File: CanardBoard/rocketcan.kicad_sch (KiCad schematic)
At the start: 18 parts, among them J10 G125-MH104M4-04AD000P, U13 TCAN3413DDFR, U14 TPS2521

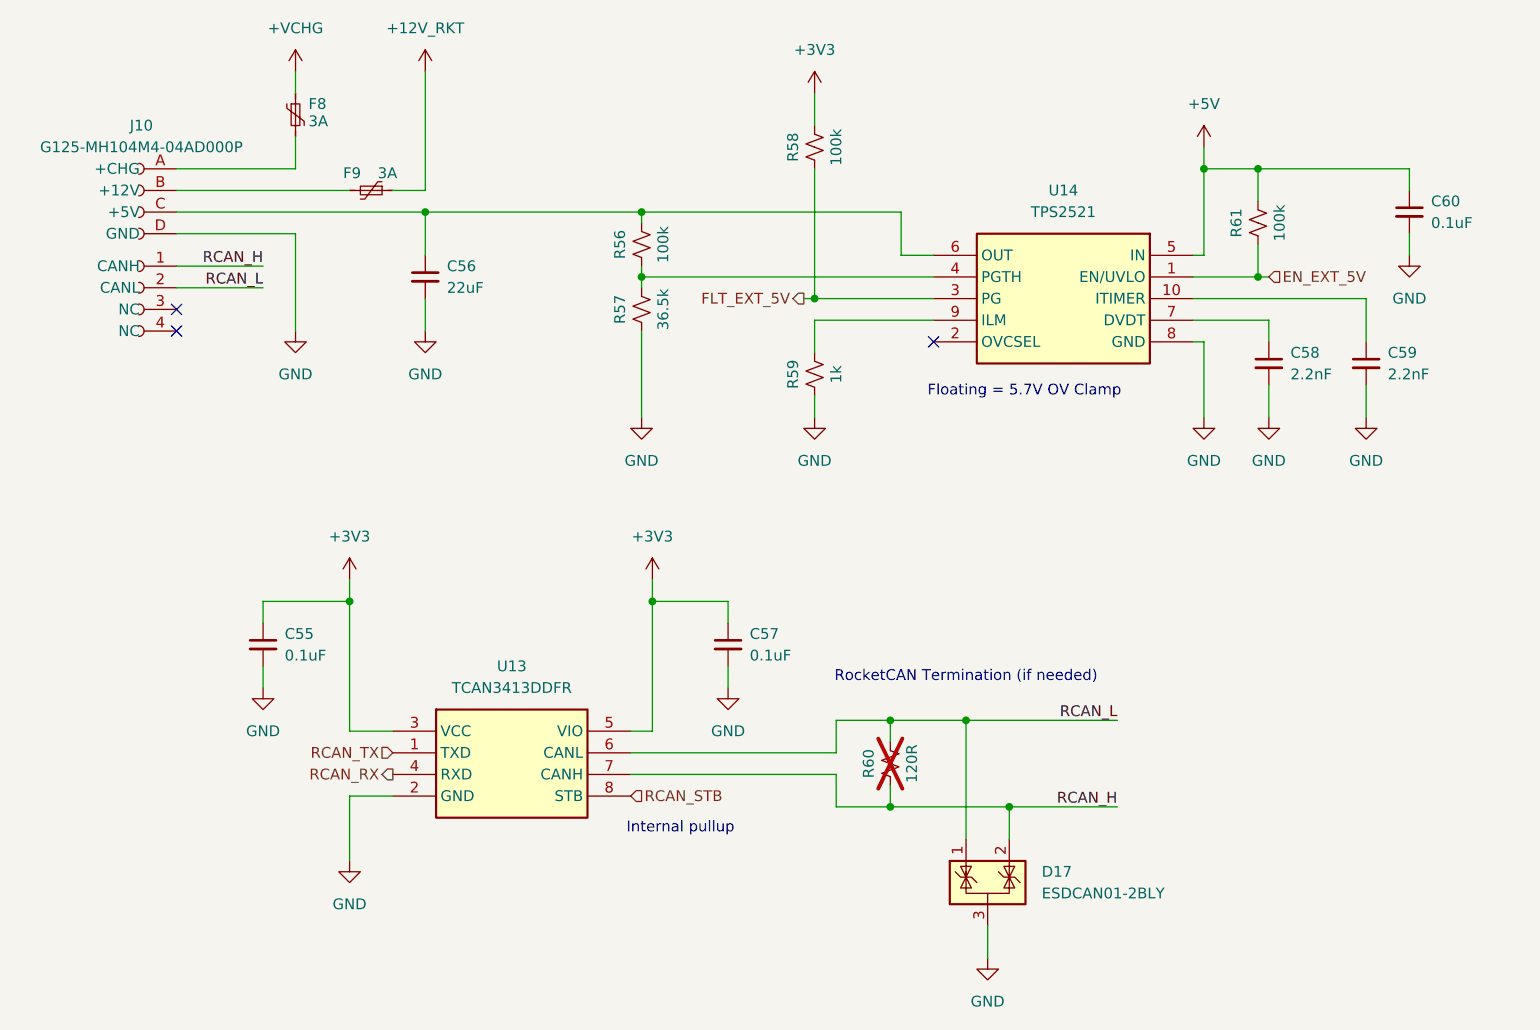
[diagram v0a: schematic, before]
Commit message: stuff
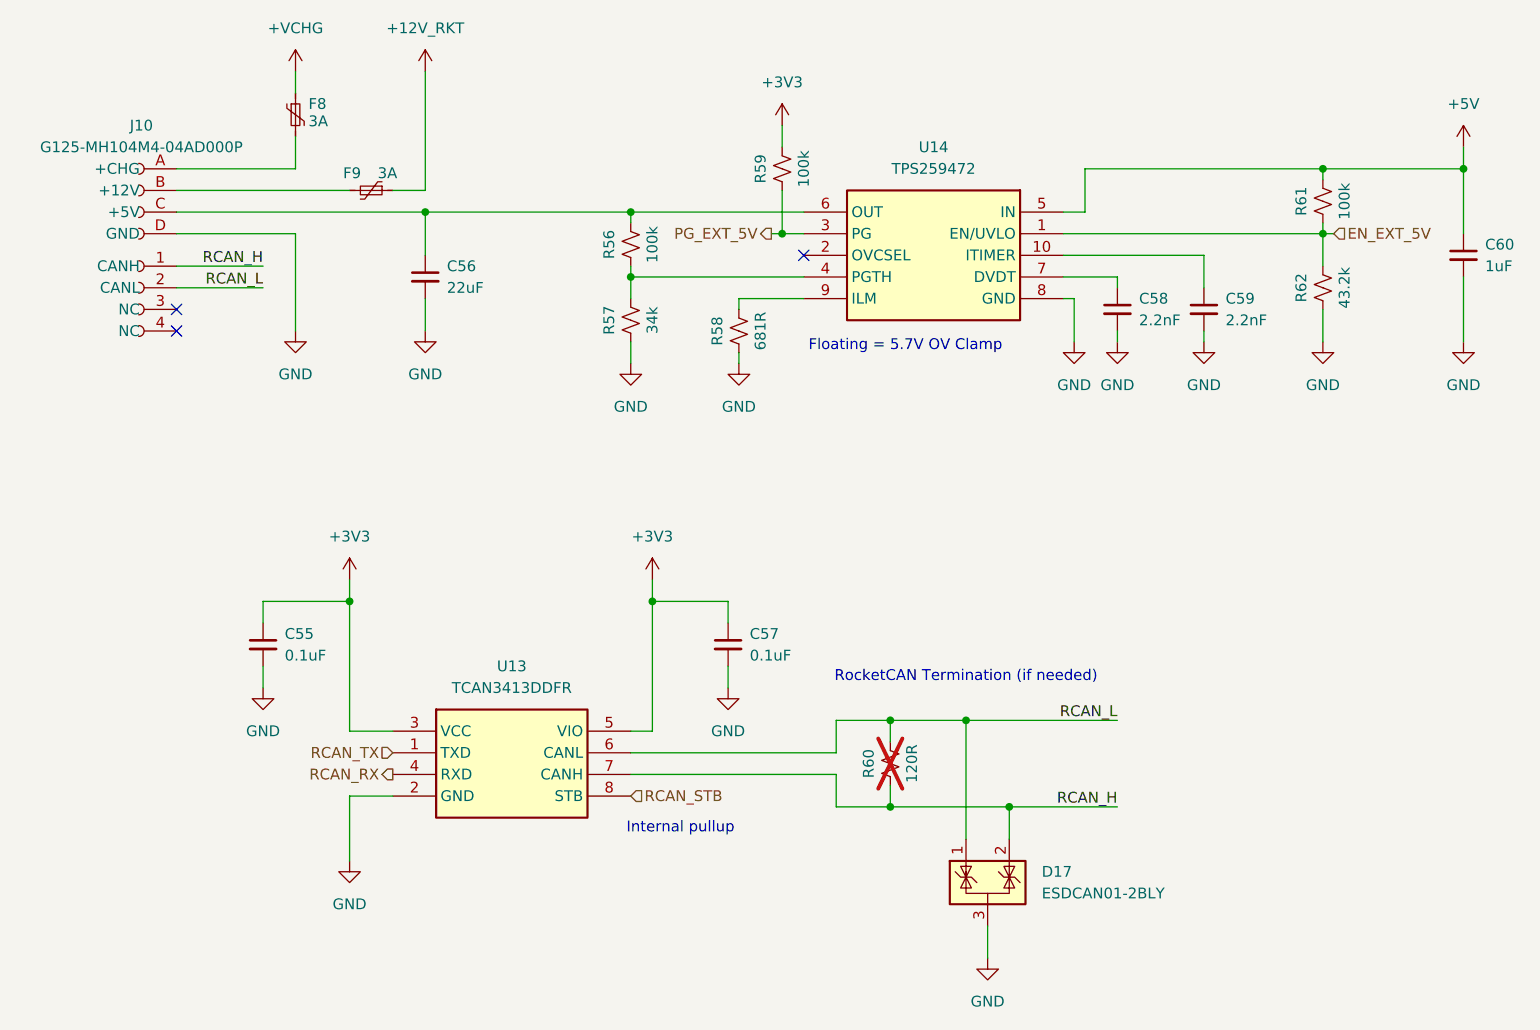
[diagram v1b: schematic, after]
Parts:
- removed U14: TPS2521, canardboard:TPS2521, symbol canardboard:TPS2521
- added R62: 43.2k, Resistor_SMD:R_0402_1005Metric, symbol Device:R_Small_US
- added U14: TPS259472, canardboard:TPS25947xx, symbol canardboard:TPS259472
- C60: value 0.1uF -> 1uF
- R57: value 36.5k -> 34k
- R58: value 100k -> 681R
- R59: value 1k -> 100k
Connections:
- net FLT_EXT_5V is gone; now on net GND: R58.2
- net +3V3: now also R59.1; no longer R58.1
- net +5V: now also U14.5 (IN)
- net EN_EXT_5V: now also R62.1, U14.1 (EN/UVLO)
- net GND: now also R62.2, U14.8 (GND); no longer R59.2
- net at C59.1: now also U14.10 (ITIMER)
- net at C56.1, J10.C (+5V), R56.1: now also U14.6 (OUT)
- net at R56.2, R57.1: now also U14.4 (PGTH)
- net at C58.1: now also U14.7 (DVDT)
- new net: R58.1, U14.9 (ILM)
- new net PG_EXT_5V: R59.2, U14.3 (PG)
